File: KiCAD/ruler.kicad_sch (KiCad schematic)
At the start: 64 parts, among them J1 ICP6, U1 ATtiny85V-10SU

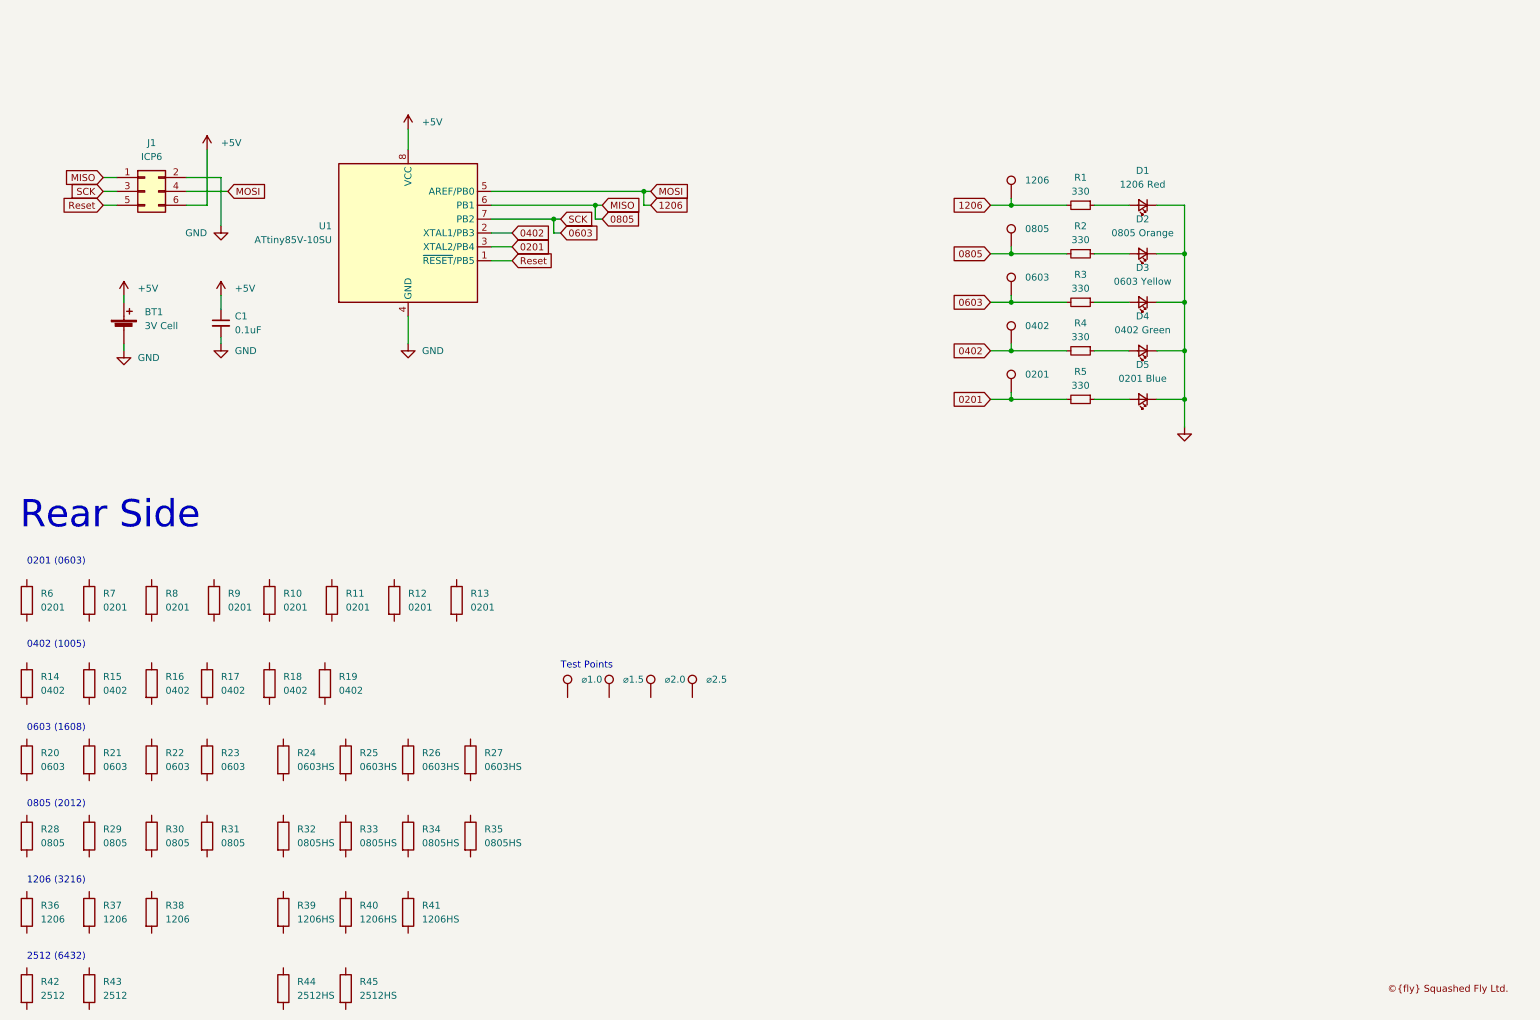
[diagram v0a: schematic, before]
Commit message: update
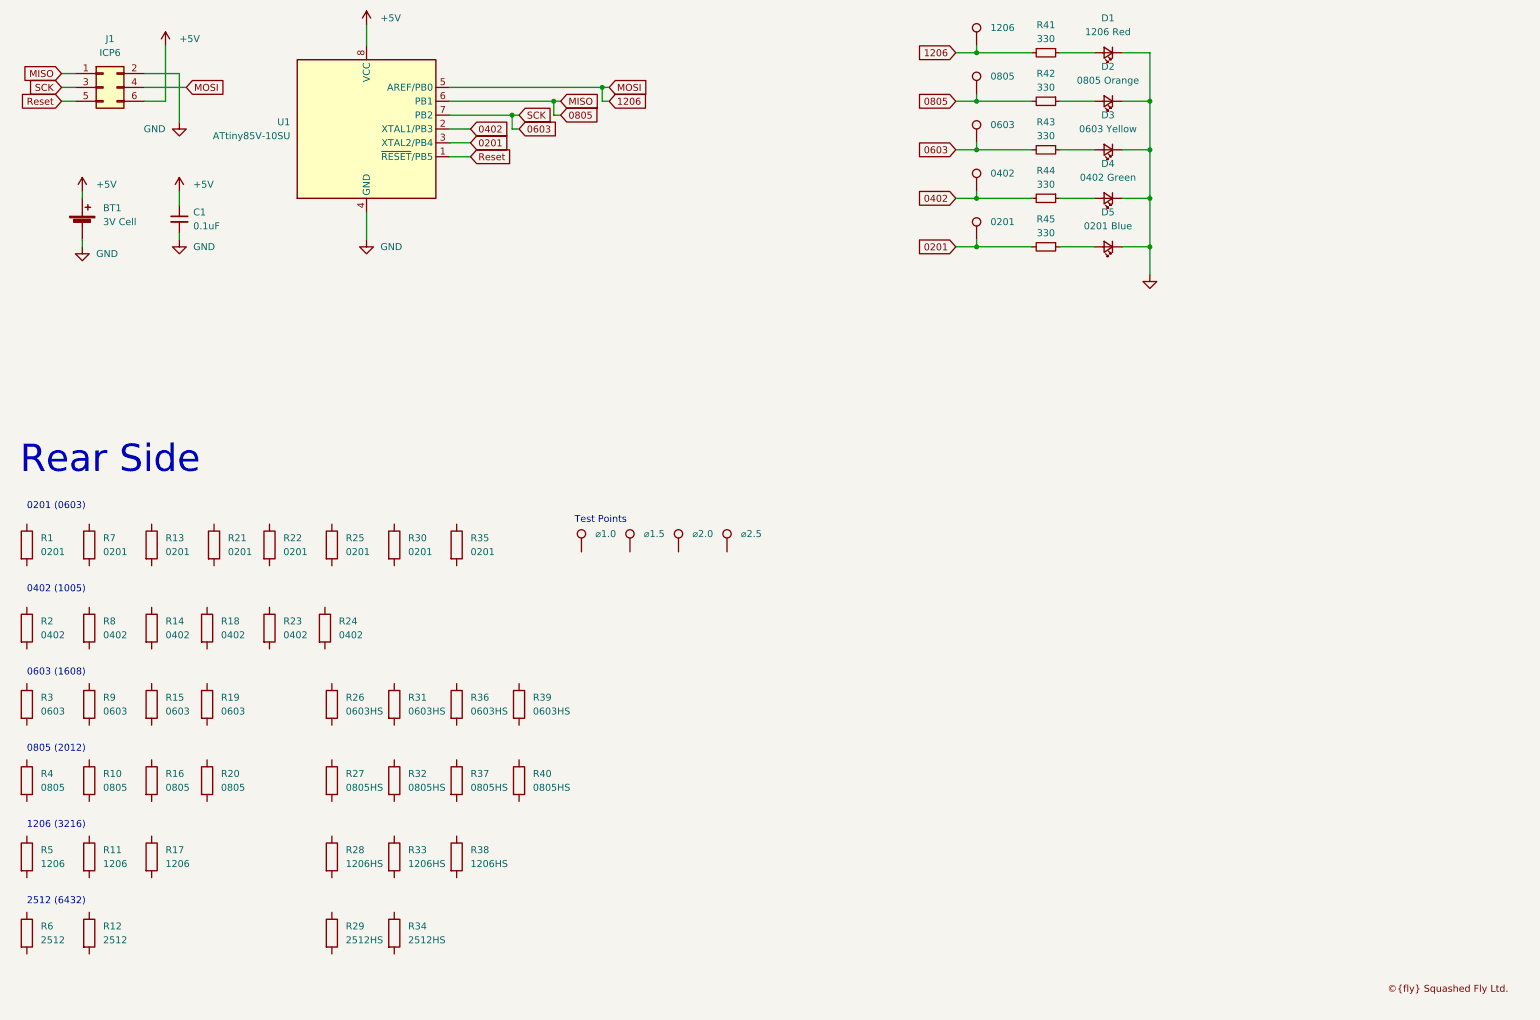
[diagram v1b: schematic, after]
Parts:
- R26: renamed from R24; footprint Resistor_SMD:R_0603_1608Metric_Pad1.05x0.95mm_HandSolder -> Resistor_SMD:R_0603_1608Metric_Pad0.98x0.95mm_HandSolder
- R27: renamed from R32; footprint Resistor_SMD:R_0805_2012Metric_Pad1.15x1.40mm_HandSolder -> Resistor_SMD:R_0805_2012Metric_Pad1.20x1.40mm_HandSolder
- R28: renamed from R39; footprint Resistor_SMD:R_1206_3216Metric_Pad1.42x1.75mm_HandSolder -> Resistor_SMD:R_1206_3216Metric_Pad1.30x1.75mm_HandSolder
- R29: renamed from R44; footprint Resistor_SMD:R_2512_6332Metric_Pad1.52x3.35mm_HandSolder -> Resistor_SMD:R_2512_6332Metric_Pad1.40x3.35mm_HandSolder
- R31: renamed from R25; footprint Resistor_SMD:R_0603_1608Metric_Pad1.05x0.95mm_HandSolder -> Resistor_SMD:R_0603_1608Metric_Pad0.98x0.95mm_HandSolder
- R32: renamed from R33; footprint Resistor_SMD:R_0805_2012Metric_Pad1.15x1.40mm_HandSolder -> Resistor_SMD:R_0805_2012Metric_Pad1.20x1.40mm_HandSolder
- R33: renamed from R40; footprint Resistor_SMD:R_1206_3216Metric_Pad1.42x1.75mm_HandSolder -> Resistor_SMD:R_1206_3216Metric_Pad1.30x1.75mm_HandSolder
- R34: renamed from R45; footprint Resistor_SMD:R_2512_6332Metric_Pad1.52x3.35mm_HandSolder -> Resistor_SMD:R_2512_6332Metric_Pad1.40x3.35mm_HandSolder
- R36: renamed from R26; footprint Resistor_SMD:R_0603_1608Metric_Pad1.05x0.95mm_HandSolder -> Resistor_SMD:R_0603_1608Metric_Pad0.98x0.95mm_HandSolder
- R37: renamed from R34; footprint Resistor_SMD:R_0805_2012Metric_Pad1.15x1.40mm_HandSolder -> Resistor_SMD:R_0805_2012Metric_Pad1.20x1.40mm_HandSolder
- R38: renamed from R41; footprint Resistor_SMD:R_1206_3216Metric_Pad1.42x1.75mm_HandSolder -> Resistor_SMD:R_1206_3216Metric_Pad1.30x1.75mm_HandSolder
- R39: renamed from R27; footprint Resistor_SMD:R_0603_1608Metric_Pad1.05x0.95mm_HandSolder -> Resistor_SMD:R_0603_1608Metric_Pad0.98x0.95mm_HandSolder
- R40: renamed from R35; footprint Resistor_SMD:R_0805_2012Metric_Pad1.15x1.40mm_HandSolder -> Resistor_SMD:R_0805_2012Metric_Pad1.20x1.40mm_HandSolder
- R42: renamed from R2; footprint Resistor_SMD:R_0805_2012Metric_Pad1.15x1.40mm_HandSolder -> Resistor_SMD:R_0805_2012Metric_Pad1.20x1.40mm_HandSolder
- R43: renamed from R3; footprint Resistor_SMD:R_0603_1608Metric_Pad1.05x0.95mm_HandSolder -> Resistor_SMD:R_0603_1608Metric_Pad0.98x0.95mm_HandSolder
- renumbered R6 to R1, R29 to R10, R37 to R11, R43 to R12, R8 to R13, R16 to R14, R22 to R15, R30 to R16, R38 to R17, R17 to R18, R23 to R19, R14 to R2, R31 to R20, R9 to R21, R10 to R22, R18 to R23, R19 to R24, R11 to R25, R20 to R3, R12 to R30, R13 to R35, R28 to R4, R1 to R41, R4 to R44, R5 to R45, R36 to R5, R42 to R6, R15 to R8, R21 to R9, TP6 to TP1, TP7 to TP2, TP8 to TP3, tp1 to TP4, TP1 to TP5, TP2 to TP6, TP3 to TP7, TP4 to TP8, TP5 to TP9
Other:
- moved on the sheet: BT1, C1, D1, D2, D3, D4, D5, J1, R1, R10, R11, R12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
